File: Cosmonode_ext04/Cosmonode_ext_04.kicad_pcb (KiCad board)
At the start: 2 copper layers, 19.7 x 31.1 mm, 24 parts, among them J1 PT100, J2 CONN_01X07, J3 CONN_01X07, J4 GS3, J5 GS3, U1 TL431ACDBZR, U2 LMV321, U3 RT9193-30PB

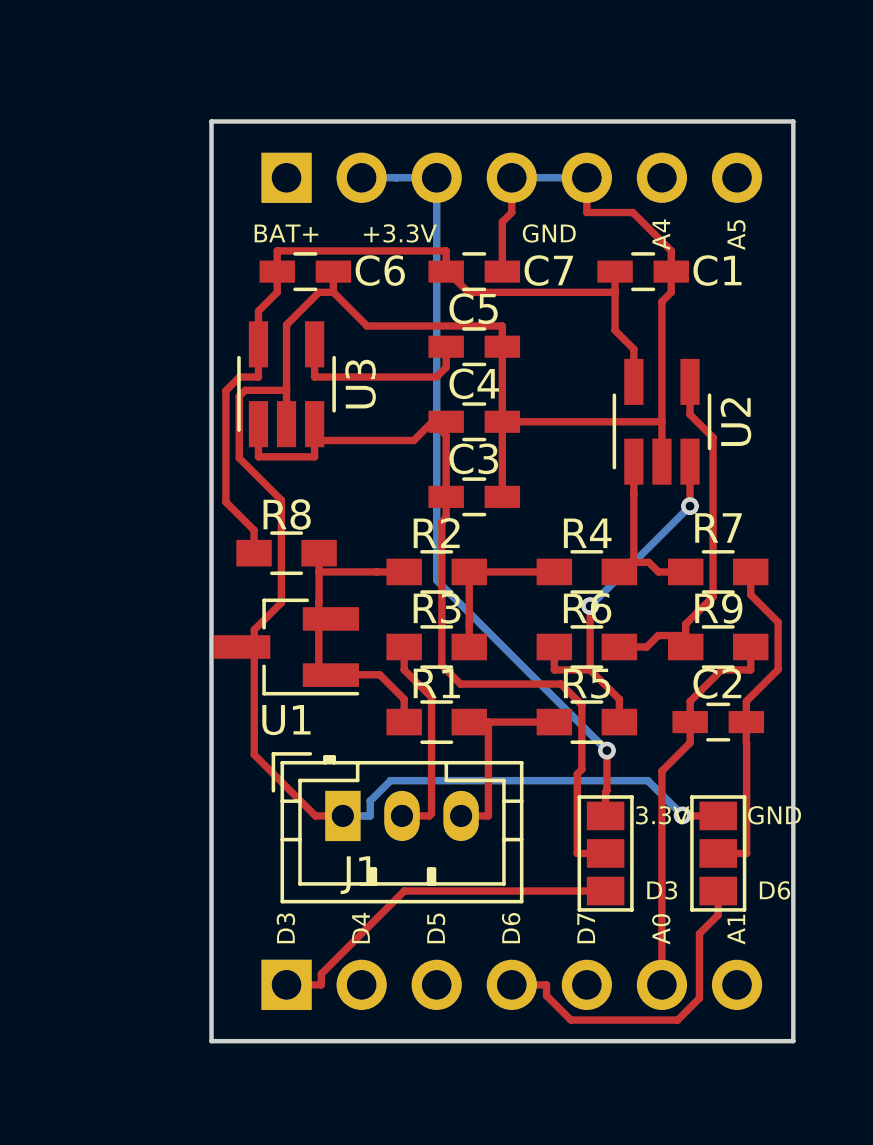
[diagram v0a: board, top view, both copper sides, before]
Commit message: fully update to v0.3
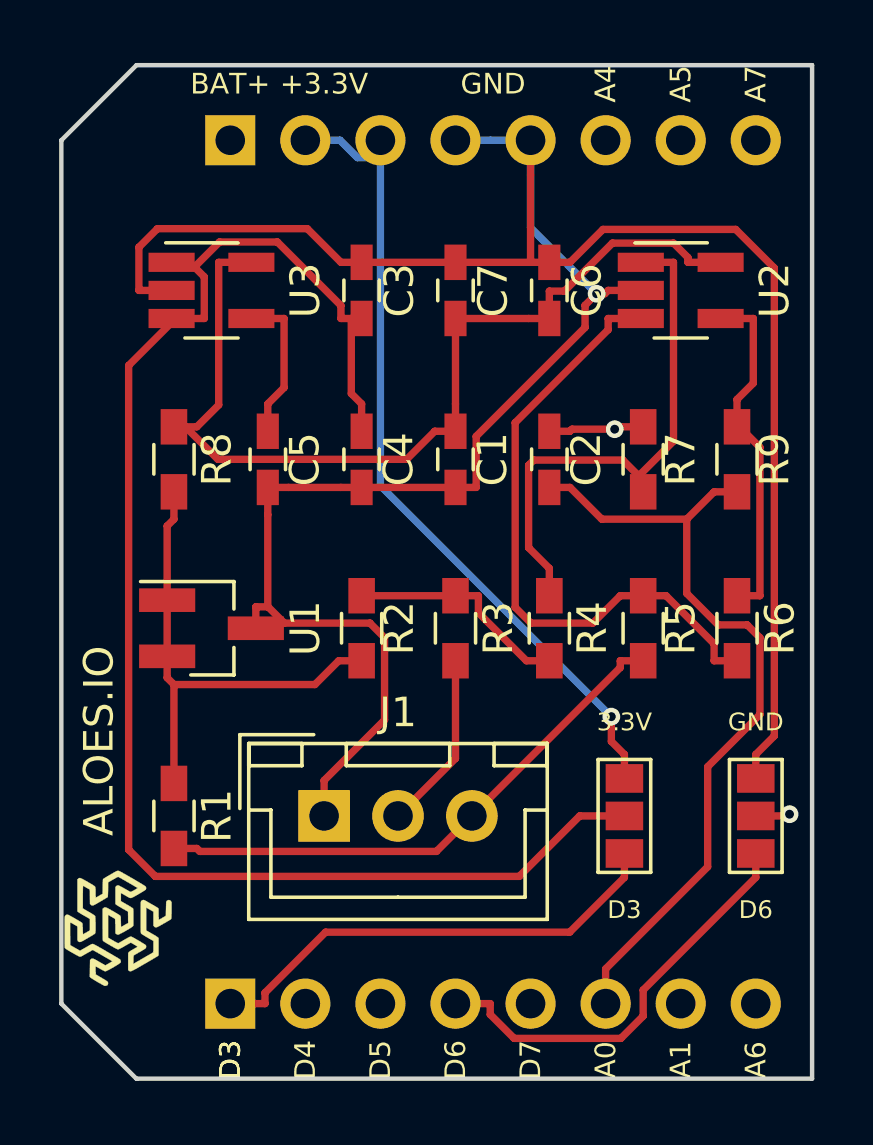
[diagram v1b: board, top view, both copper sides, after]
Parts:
- added J6: Aloes_Logo, Aloes:Aloes_mini, F.Cu at (140.3, 118.7)
- added J7: OSHW_Logo, Symbols:OSHW-Logo_5.7x6mm_SilkScreen, B.Cu at (143.5, 98.4)
- J1: footprint Connectors_JST:JST_PH_B3B-PH-K_03x2.00mm_Straight -> Connectors_JST:JST_XH_B03B-XH-A_03x2.50mm_Straight
- J2, J3: value CONN_01X07 -> CONN_01X08; footprint Pin_Headers:Pin_Header_Straight_1x07_Pitch2.54mm -> Socket_Strips:Socket_Strip_Straight_1x08_Pitch2.54mm
- moved C2 10.6 mm to (154.9, 102.9), turned to 270 degrees
- moved R1 9.44 mm to (142.2, 114.9), turned to 270 degrees
- moved C1 8.98 mm to (151.8, 102.9), turned to 270 degrees
- moved C6 8.28 mm to (154.9, 97.2), turned to 90 degrees
- moved C5 7.96 mm to (145.4, 102.9), turned to 270 degrees
- moved C3 7.96 mm to (148.6, 97.2), turned to 90 degrees
- moved R9 6.38 mm to (161.3, 102.9), turned to 90 degrees
- moved R6 5.12 mm to (161.3, 108.6), turned to 270 degrees
- moved R8 4.96 mm to (142.2, 102.9), turned to 270 degrees
- moved R7 4.58 mm to (158.1, 102.9), turned to 90 degrees
- moved U2 4.49 mm to (159.4, 97.2), turned to 0 degrees
- moved U3 4.07 mm to (143.5, 97.2), turned to 0 degrees
- moved C4 4.02 mm to (148.6, 102.9), turned to 270 degrees
- moved R5 3.70 mm to (158.1, 108.6), turned to 90 degrees
- moved R2 3.17 mm to (148.6, 108.6), turned to 90 degrees
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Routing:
- net Net-(C3-Pad1): track 28.7 -> 51.7 mm
- net GND: track 73.8 -> 89.4 mm
- net /A0: track 13.3 -> 27.3 mm
- net Net-(R4-Pad1): track 5.92 -> 18.1 mm
- net Net-(J1-Pad3): track 6.98 -> 18.7 mm
- net Net-(R5-Pad2): track 12.6 -> 21.5 mm, vias 2 -> 0
- net Net-(C2-Pad1): track 11.3 -> 4.40 mm, vias 0 -> 2
- net /+2.495V: track 11.0 -> 16.7 mm
- net /+3.0V: track 28.1 -> 32.5 mm
- net /D3: track 12.3 -> 16.1 mm
- net /D6: track 11.3 -> 14.4 mm
- net Net-(R2-Pad2): track 5.42 -> 7.60 mm
- net VCC: track 26.5 -> 27.8 mm
- net Net-(C5-Pad1): track 6.39 -> 5.15 mm
- net Net-(J1-Pad2): track 7.05 -> 6.06 mm
- added copper zone on B.Cu, net Net-(C2-Pad1)
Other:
- board size 19.7 x 31.1 mm -> 25.4 x 34.3 mm
- board text added: "A6"
- board text added: "A7"
- board text added: "ALOES.IO"
- board text added: "Extension #4 PT100 driver"
- board text removed: "Cosmonode PT100 driver"
